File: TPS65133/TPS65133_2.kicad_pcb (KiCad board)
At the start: 2 copper layers, 19.8 x 50.3 mm, 16 parts, among them U1 TPS65133DPDR

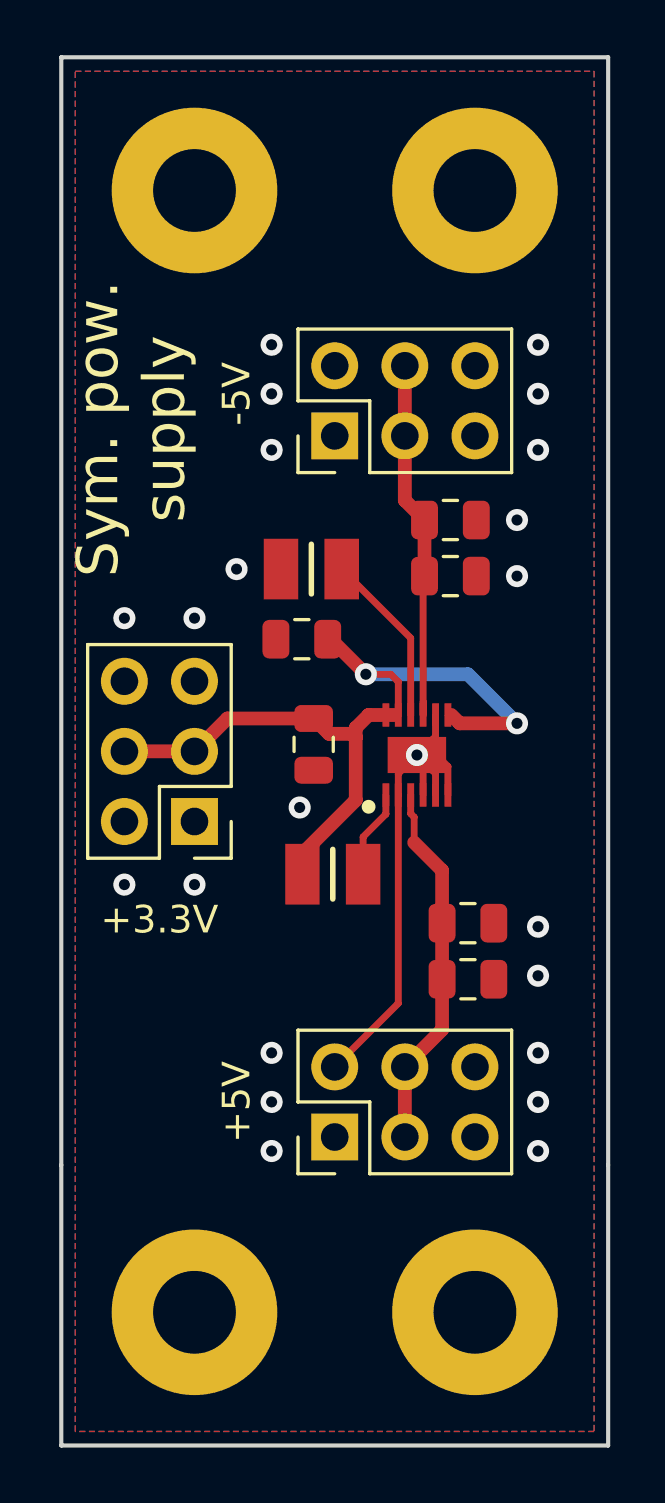
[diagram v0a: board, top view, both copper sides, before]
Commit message: New components
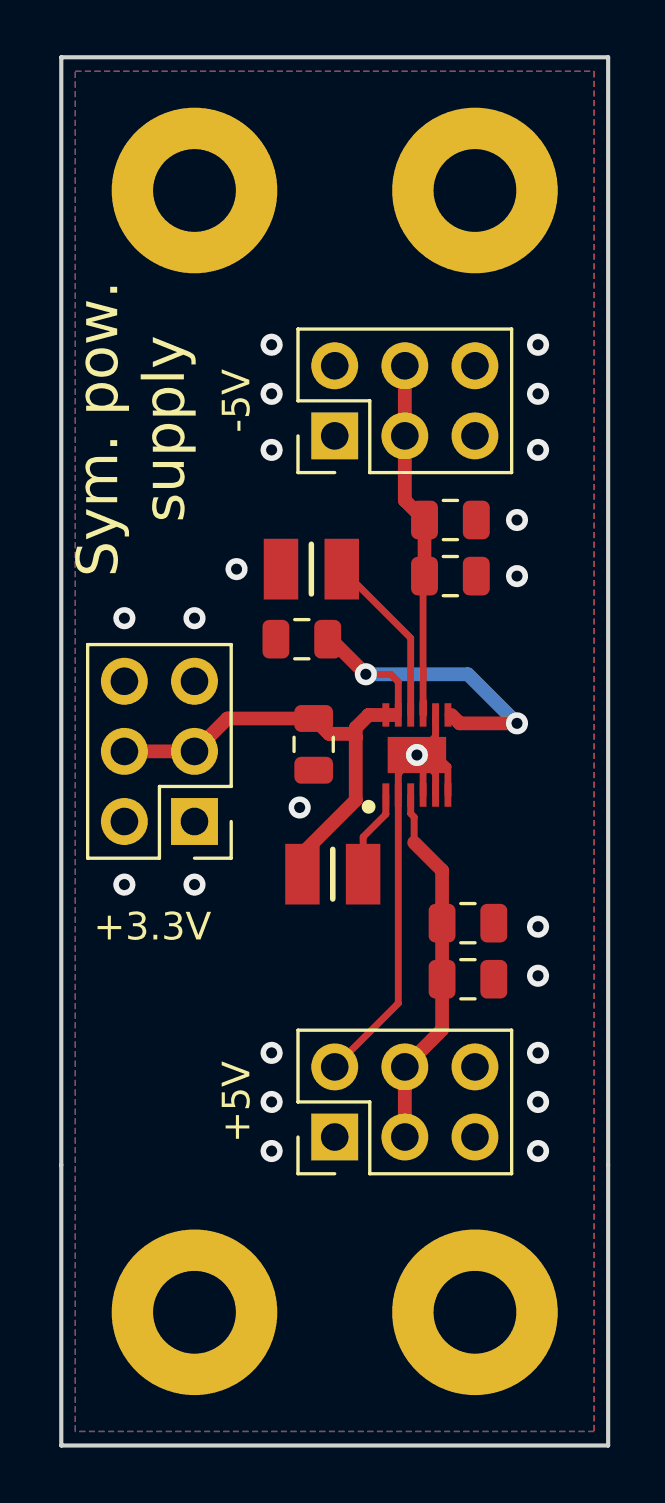
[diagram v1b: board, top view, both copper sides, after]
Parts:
- +3.3V, +5V, -5V: value (none) -> 02x03_Male
- C1, C5, C6: value GRM21BR71E104KA01 -> (none)
- C2: value GRM21BR71A106KE51 -> (none)
- C3, C4: value GRM21BR71A106KE5 -> (none)
- L1, L2: value 1239AS-H-4R7M=P2 -> (none)
- U1: value TPS65133DPDR -> (none)
